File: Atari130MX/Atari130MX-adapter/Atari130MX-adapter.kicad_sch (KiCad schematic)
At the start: 9 parts, among them J0 Conn_01x24, J1 Conn_01x24, J2 Conn_01x26, J3 Conn_02x12_Odd_Even, J4 Conn_01x24, J5 Conn_01x26, J6 Conn_02x12_Odd_Even, J7 Conn_01x24, J8 Conn_01x26

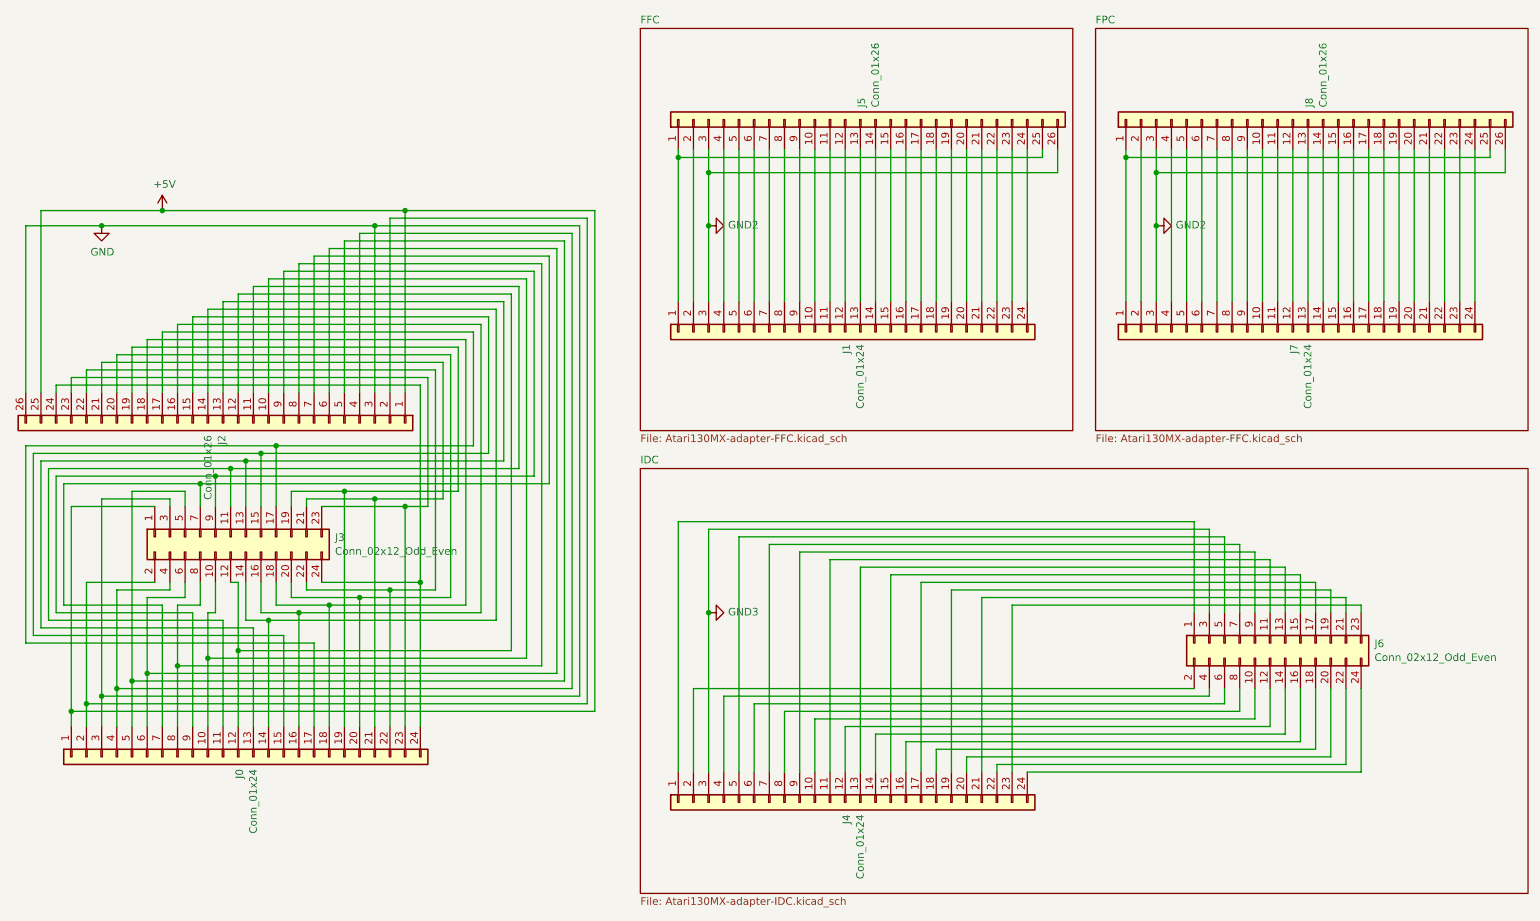
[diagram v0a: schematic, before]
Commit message: Revised adapter
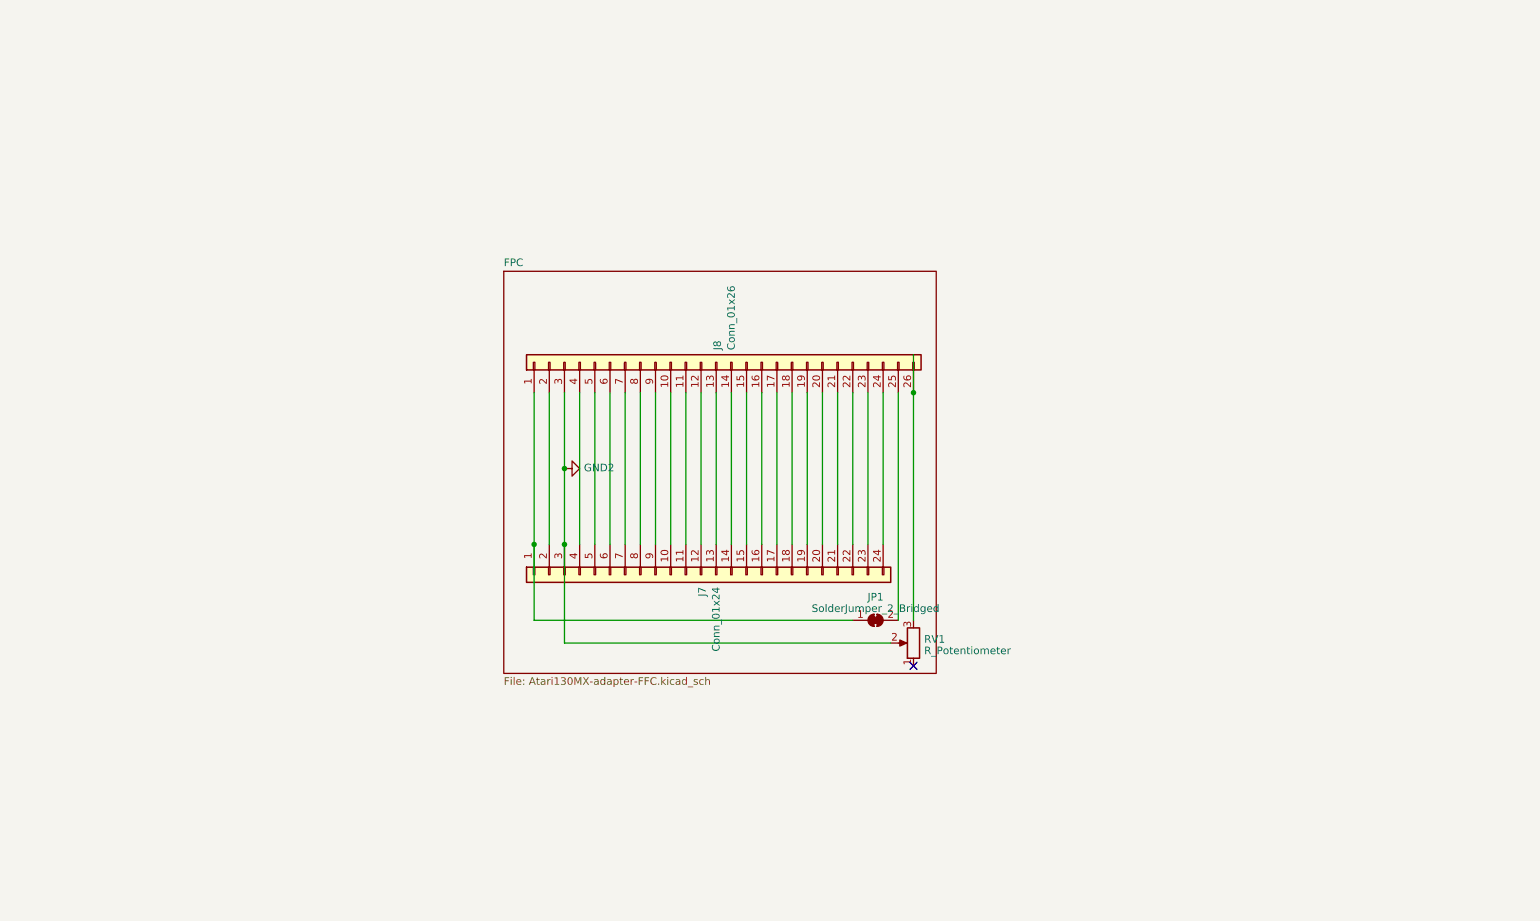
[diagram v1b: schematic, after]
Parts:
- removed J0, J1, J4: Conn_01x24, Atari130MX:1x24_P1.27mm_Edge_Back, symbol Connector_Generic:Conn_01x24
- removed J2, J5: Conn_01x26, Connector_FFC-FPC:Molex_200528-0260_1x26-1MP_P1.00mm_Horizontal, symbol Connector_Generic:Conn_01x26
- removed J3, J6: Conn_02x12_Odd_Even, Connector_IDC:IDC-Header_2x12_P2.54mm_Vertical, symbol Connector_Generic:Conn_02x12_Odd_Even
- added JP1: SolderJumper_2_Bridged, Jumper:SolderJumper-2_P1.3mm_Bridged_RoundedPad1.0x1.5mm, symbol Jumper:SolderJumper_2_Bridged
- added RV1: R_Potentiometer, Atari130MX:Potentiometer_CUI-PTN06-D02CB20, symbol Device:R_Potentiometer
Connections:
- net GND2: now also RV1.2; no longer J8.26 (Pin_26)
- net at J7.1 (Pin_1), J8.1 (Pin_1): now also JP1.1 (A); no longer J8.25 (Pin_25)
- new net: J8.26 (Pin_26), RV1.3
- new net: J8.25 (Pin_25), JP1.2 (B)
- no-connect marks 0 -> 1
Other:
- removed sheet FFC
- removed sheet IDC
- moved on the sheet: J7, J8

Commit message: Sideways XE adapter
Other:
- title: Atari XEMX keyboard adapter -> Atari XE keyboard adapter
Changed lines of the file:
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@@
   (paper "A4")
   (title_block
-    (title "Atari XEMX keyboard adapter")
-    (date "2021-09-19")
-    (rev "A")
+    (title "Atari XE keyboard adapter")
+    (date "2023-03-31")
+    (rev "F")
     (company "Decent Consulting")
   )
